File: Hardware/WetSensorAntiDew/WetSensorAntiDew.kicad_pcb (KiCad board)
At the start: 2 copper layers, 96.5 x 104.1 mm, 30 parts, among them J2 Connector to BME280, J3 4P4C, J5 Connector to power supply, J6 Conn_01x04_Socket, J8 6P6C, Q1 MOSFET N-CH, SW1 SW_Push, U1 AMS1117, U3 STM32F103C6Tx, Y1 Crystal_GND24_Small

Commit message: finished pcb layout
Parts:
- removed JP1: SolderJumper_3_Bridged12, Jumper:SolderJumper-3_P1.3mm_Bridged12_Pad1.0x1.5mm_NumberLabels
- added C7: C, Capacitor_SMD:C_0603_1608Metric_Pad1.08x0.95mm_HandSolder, F.Cu at (108.2, 115.1)
- J2: footprint Connector_PinSocket_2.54mm:PinSocket_1x04_P2.54mm_Horizontal -> Connector_PinSocket_2.54mm:PinSocket_1x05_P2.54mm_Horizontal; moved to F.Cu
- J5: footprint Connector_Phoenix_MSTB:PhoenixContact_MSTBA_2,5_2-G_1x02_P5.00mm_Horizontal -> Connector_Phoenix_MC:PhoenixContact_MC_1,5_2-G-3.81_1x02_P3.81mm_Horizontal
- R7: value 10k -> 1.5k
- moved D1 63.5 mm to (100.3, 110.7), turned to 90 degrees
- moved R7 58.9 mm to (104.6, 103.7), turned to -90 degrees
- moved R4 56.5 mm to (117.2, 115.7), turned to 90 degrees
- moved U2 56.1 mm to (103.5, 111.4), turned to 180 degrees
- moved JP3 55.0 mm to (94.5, 114.2), turned to 90 degrees
- moved C1 52.6 mm to (106.5, 110.9), turned to 90 degrees
- moved C2 52.2 mm to (98.6, 110.6), turned to 90 degrees
- moved R5 51.1 mm to (110.7, 111.9)
- moved C3 50.3 mm to (115.7, 114.8), turned to 90 degrees
- moved R6 48.4 mm to (108.2, 110.9), turned to -90 degrees
- moved SW1 47.9 mm to (110.3, 91.2), turned to -90 degrees
- moved R1 46.0 mm to (96.7, 110.6), turned to 90 degrees
- moved U1 45.4 mm to (112.8, 118.5), turned to 90 degrees
- moved JP2 44.4 mm to (104.3, 114.6), turned to 180 degrees
- moved R3 41.2 mm to (97.6, 108.2), turned to 180 degrees
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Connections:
- R11 pad 2: Net-(JP1-C) -> Earth
- U2 pad 13: (no net) -> Earth
- U2 pad 6: unconnected-(U2-CLMODE-Pad6) -> Earth
- U3 pad 10: PA0 -> unconnected-(U3-PA0-Pad10)
- U3 pad 29: unconnected-(U3-PA8-Pad29) -> PA0
- U3 pad 31: unconnected-(U3-PA10-Pad31) -> PIN6
- U3 pad 32: unconnected-(U3-PA11-Pad32) -> PB5
- U3 pad 41: FWD -> unconnected-(U3-PB5-Pad41)
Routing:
- net Earth: track 0.00 -> 87.3 mm, vias 0 -> 2
- net +3V3: track 0.30 -> 70.0 mm, vias 0 -> 5
- net PIN2: track 0.00 -> 34.7 mm
- net +12V: track 0.00 -> 33.8 mm
- net PIN6: track 0.00 -> 32.1 mm
- net WET1: track 0.00 -> 29.4 mm
- net WET2: track 0.00 -> 26.0 mm
- net /SWIO: track 0.00 -> 24.9 mm, vias 0 -> 1
- net /SWCLK: track 0.00 -> 20.3 mm, vias 0 -> 1
- net PB5: track 0.00 -> 19.5 mm
- net Net-(U3-NRST): track 0.00 -> 14.9 mm
- net MOSFET: track 0.00 -> 13.6 mm, vias 0 -> 1
- net Net-(U1-ADJ): track 0.00 -> 12.9 mm
- net PA0: track 0.00 -> 12.3 mm, vias 0 -> 2
- net +12C: track 0.00 -> 12.2 mm
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- added copper zone on B.Cu, net Earth
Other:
- board size 96.5 x 104.1 mm -> 37.5 x 48.6 mm

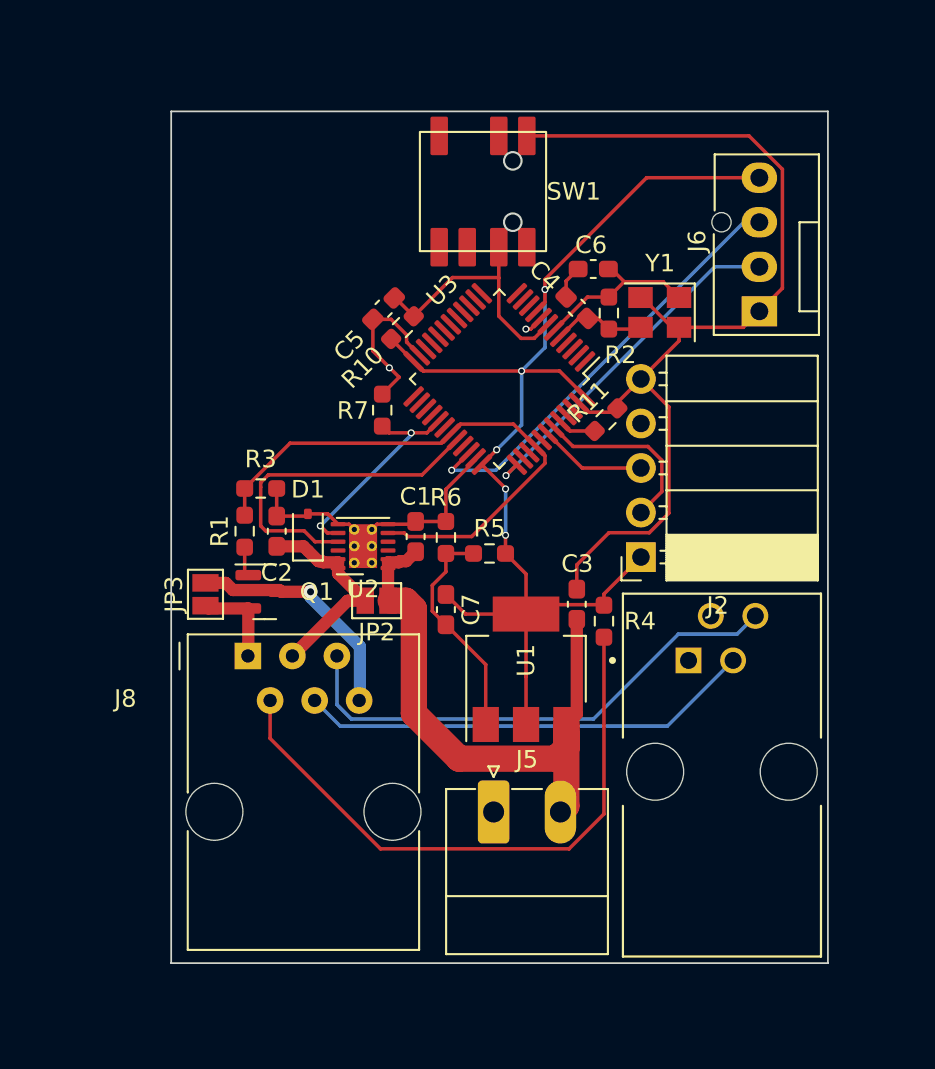
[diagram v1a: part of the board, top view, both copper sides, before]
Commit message: Final* PCB design
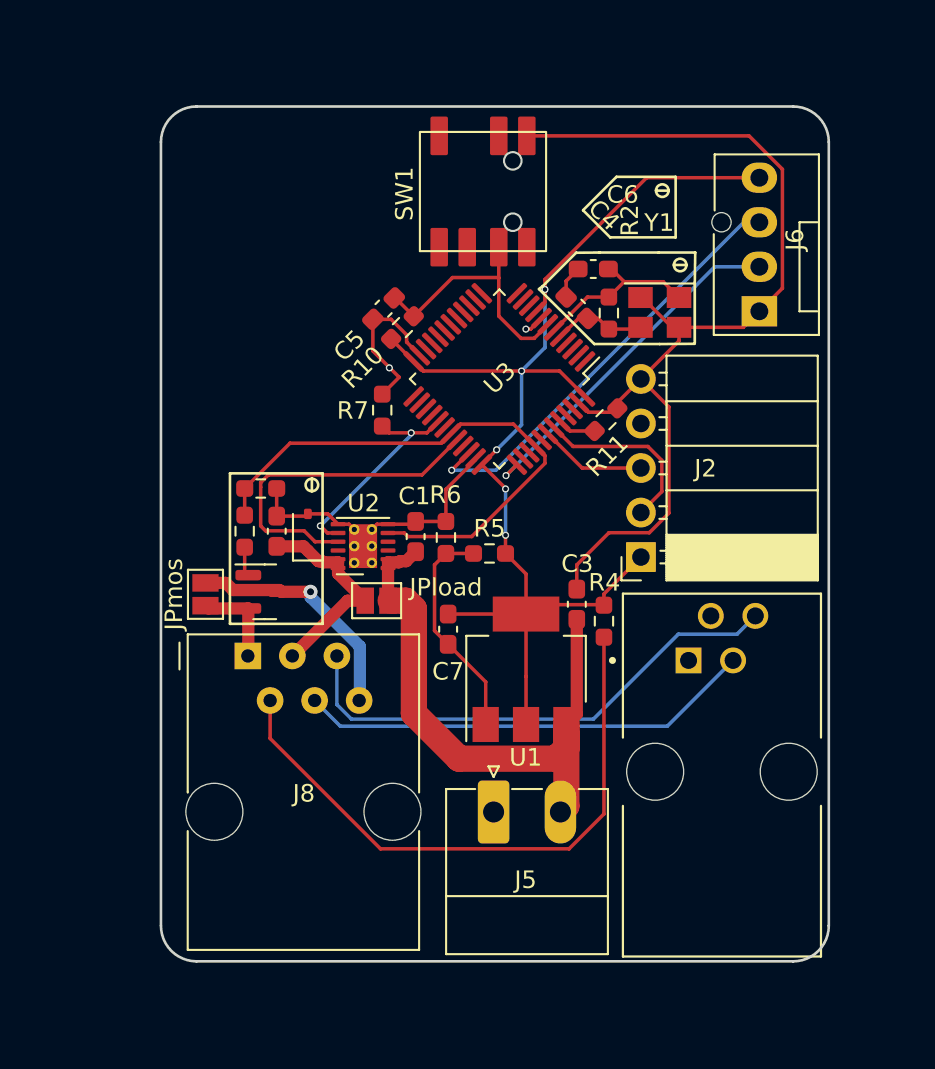
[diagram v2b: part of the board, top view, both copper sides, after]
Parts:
- moved C7 1.12 mm to (108.3, 116.2)
- renumbered JP2 to JPload, JP3 to JPmos
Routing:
- net +3V3: track 70.0 -> 69.5 mm
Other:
- board size 37.5 x 48.6 mm -> 38.1 x 48.8 mm
